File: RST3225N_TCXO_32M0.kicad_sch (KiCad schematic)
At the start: 5 parts, among them U401 T6405 R24M0

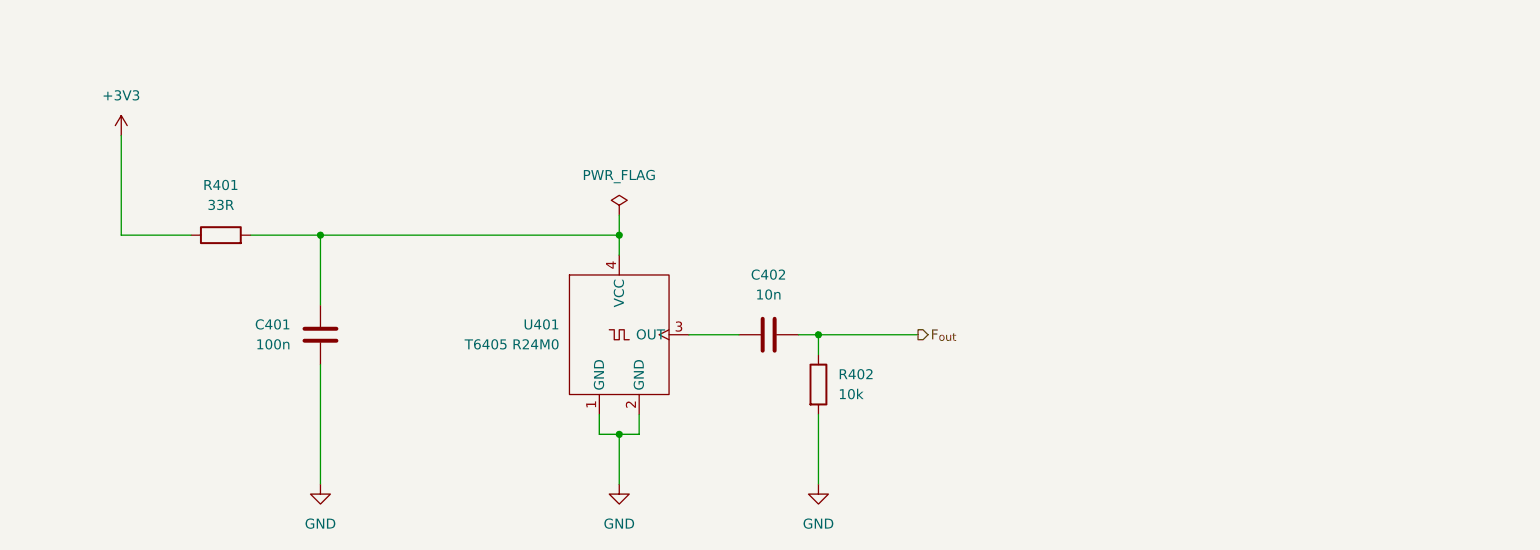
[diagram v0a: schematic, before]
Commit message: Another large revision, but we are getting closer
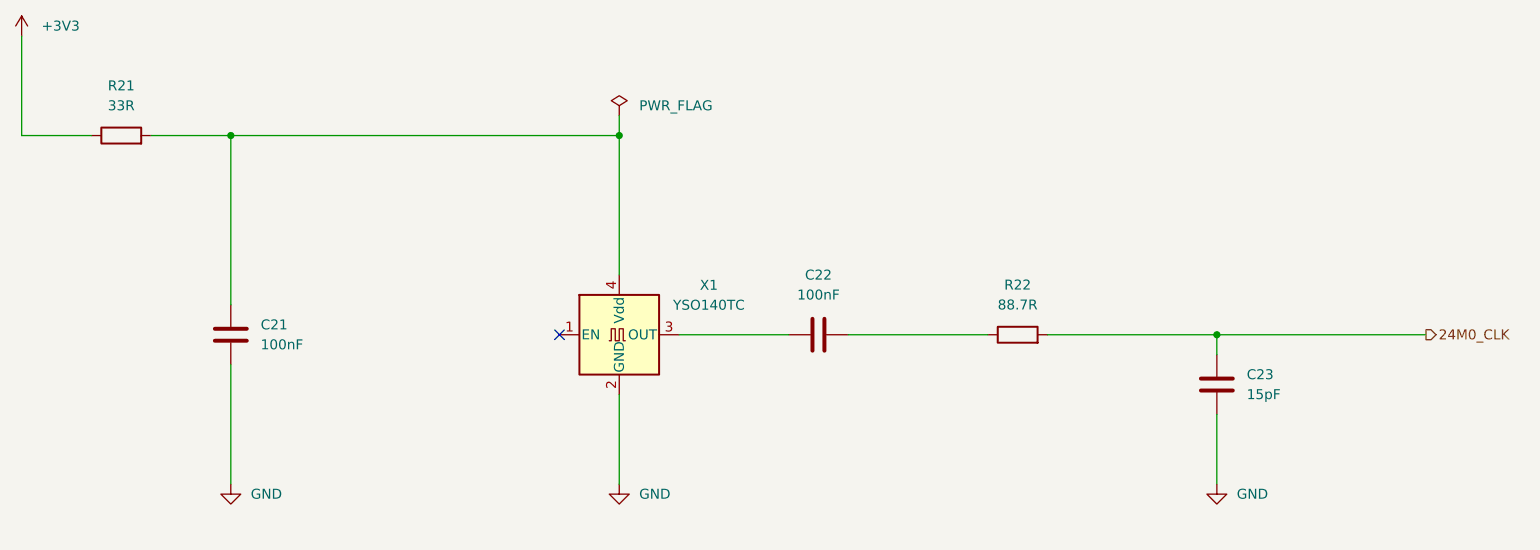
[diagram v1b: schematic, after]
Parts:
- removed U401: T6405 R24M0, cubesat_rp2040:Crystal_SMD_Rakon_3225-4Pin_3.2x2.5mm, symbol cubesat_rp2040:RST3225N
- added C23: 15pF, cubesat_rp2040:C_0402_1005Metric, symbol Device:C
- added X1: YSO140TC, cubesat_rp2040:Oscillator_SMD_YXC_YSO140TC_4Pin_3.2x2.5mm, symbol cubesat_rp2040:YSO140TC
- C21: renamed from C401; value 100n -> 100nF; LCSC_Part_Number (none) -> C960916; MANUFACTURER (none) -> Samsung Electro-Mechanics; Manufacturer_Name (none) -> Samsung Electro-Mechanics; Manufacturer_Part_Number (none) -> CL05B104KB5NNNC
- C22: renamed from C402; value 10n -> 100nF; LCSC_Part_Number (none) -> C960916; MANUFACTURER (none) -> Samsung Electro-Mechanics; Manufacturer_Name (none) -> Samsung Electro-Mechanics; Manufacturer_Part_Number (none) -> CL05B104KB5NNNC
- R21: renamed from R401; LCSC_Part_Number (none) -> C25161; Manufacturer_Name Vishay -> UNI-ROYAL(Uniroyal Elec); Manufacturer_Part_Number P-0402E33R0FGxx -> 0402WGJ0330TCE
- R22: renamed from R402; value 10k -> 88.7R; LCSC_Part_Number (none) -> C423126; Manufacturer_Name Vishay -> UNI-ROYAL(Uniroyal Elec); Manufacturer_Part_Number P-0402E1002FGxx -> 0402WGF887JTCE
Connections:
- net GND: now also C23.1, X1.2 (GND); no longer R22.2
- net at C22.1: now also X1.3 (OUT)
- net at C21.1, R21.2: now also X1.4 (Vdd)
- net F_{out}: no longer names the net of C22.2, R22.1
- new net 24M0_CLK: C23.2, R22.2
- no-connect marks 0 -> 1
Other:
- moved on the sheet: C21, C22, R21, R22
